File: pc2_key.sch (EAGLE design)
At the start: 48 parts

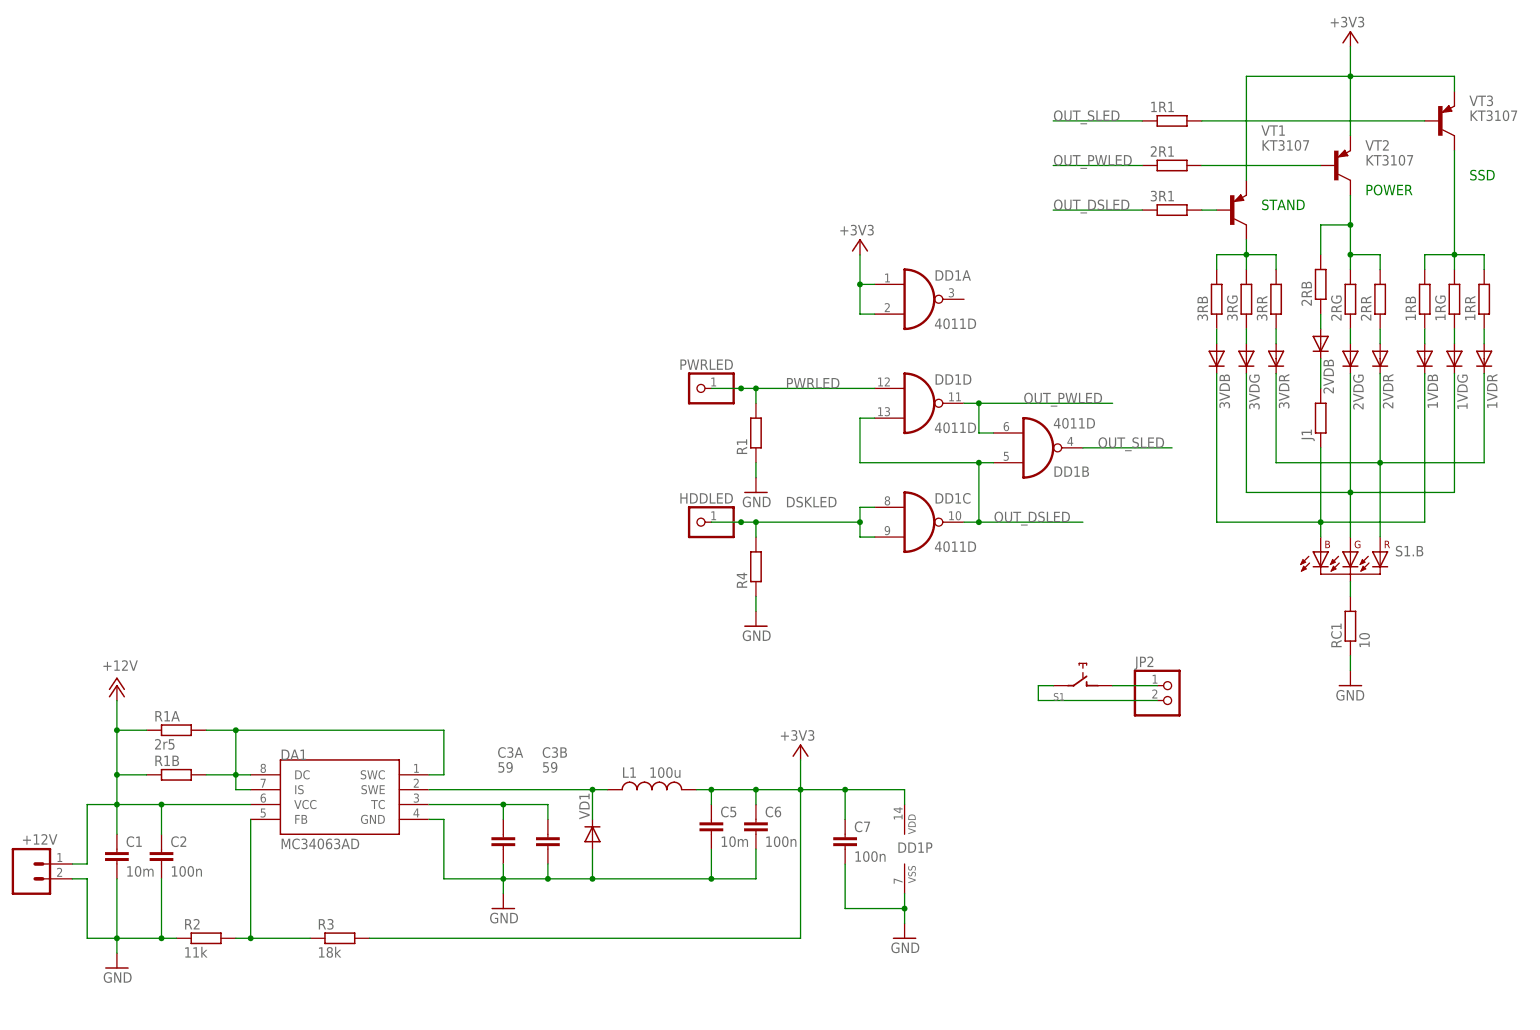
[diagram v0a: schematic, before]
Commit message: 15
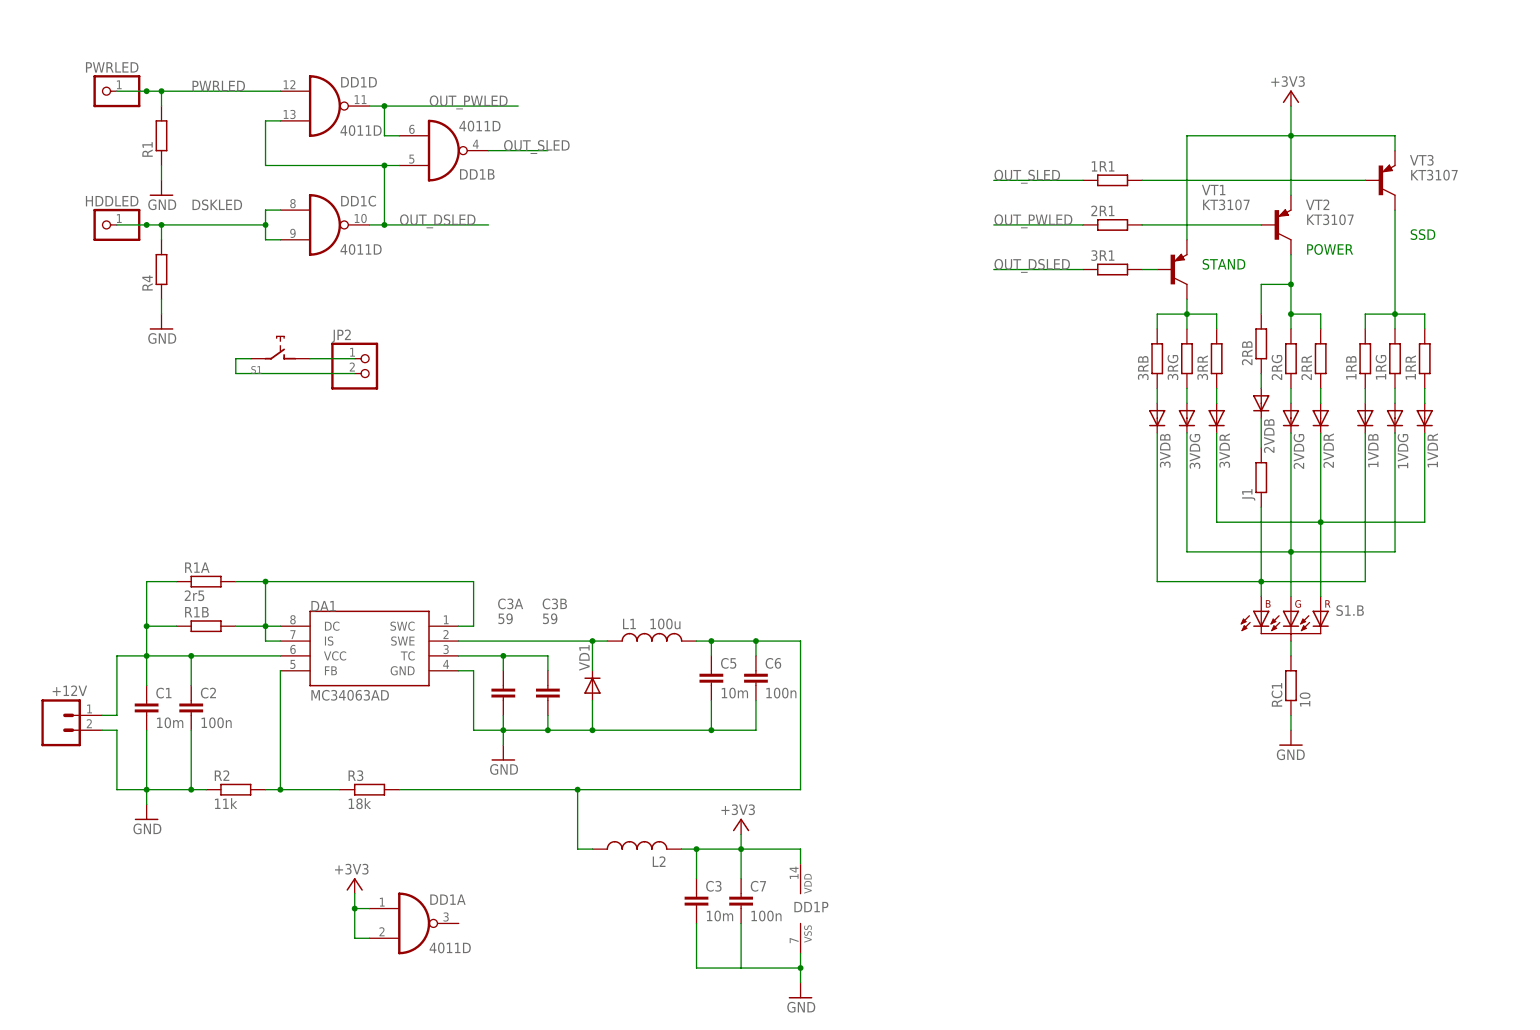
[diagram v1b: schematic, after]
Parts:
- added C3: 10m, rcl:C-EUC1210
- added L2: (no value), rcl:L-USL1812
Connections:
- net +12V renamed N$30
- new net N$29: C5.1, C6.1, L1.2, L2.1, R3.2
- net +3V3: now also C3.1, L2.2; no longer C5.1, C6.1, L1.2, R3.2
- net GND: now also C3.2
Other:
- moved on the sheet: +12V, 1R1, 1RB, 1RG, 1RR, 1VDB, 1VDG, 1VDR, 2R1, 2RB, 2RG, 2RR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
